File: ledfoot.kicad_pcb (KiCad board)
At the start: 2 copper layers, 29 x 84 mm, 24 parts, among them J1 1729144, J2 54-00167, J3 Conn_01x12_Pin, SW1 SW_Push, SW2 SW_Push, U1 MP1584EN, U2 SN74LVC1T45DBV

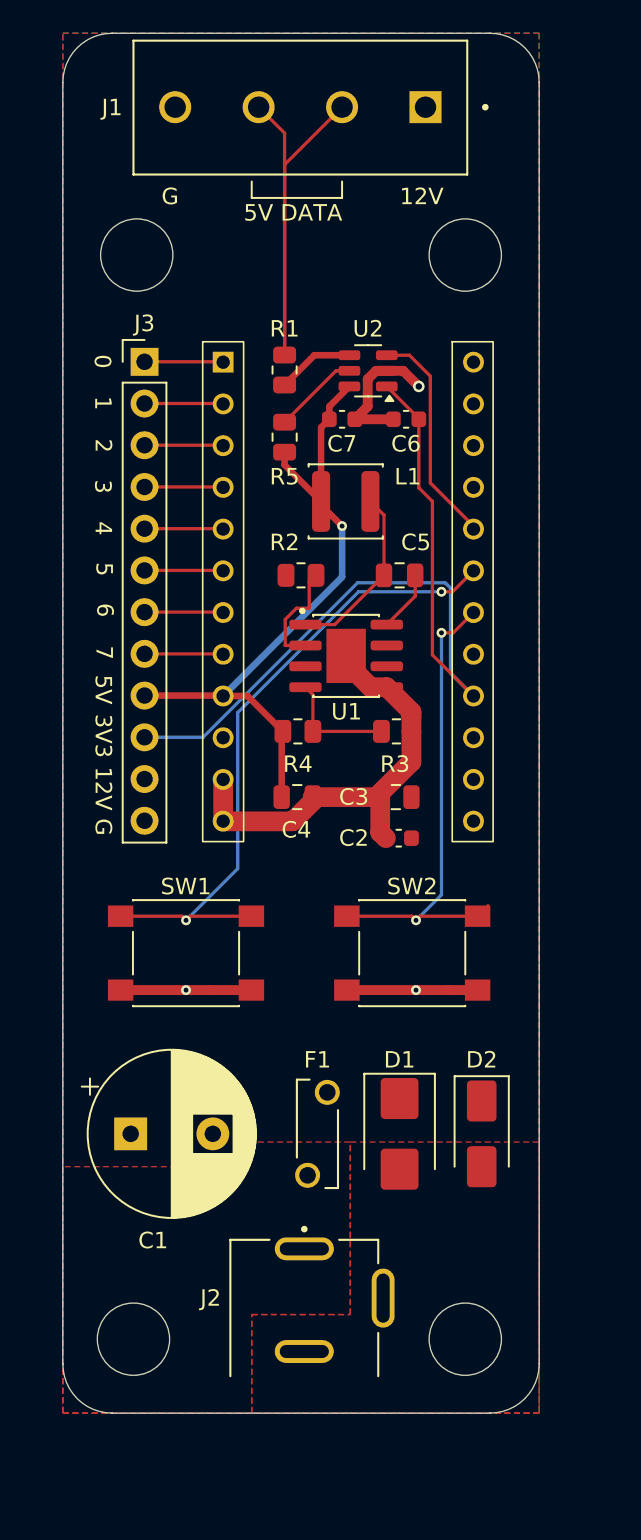
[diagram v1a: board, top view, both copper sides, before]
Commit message: Revision 2 ready for production
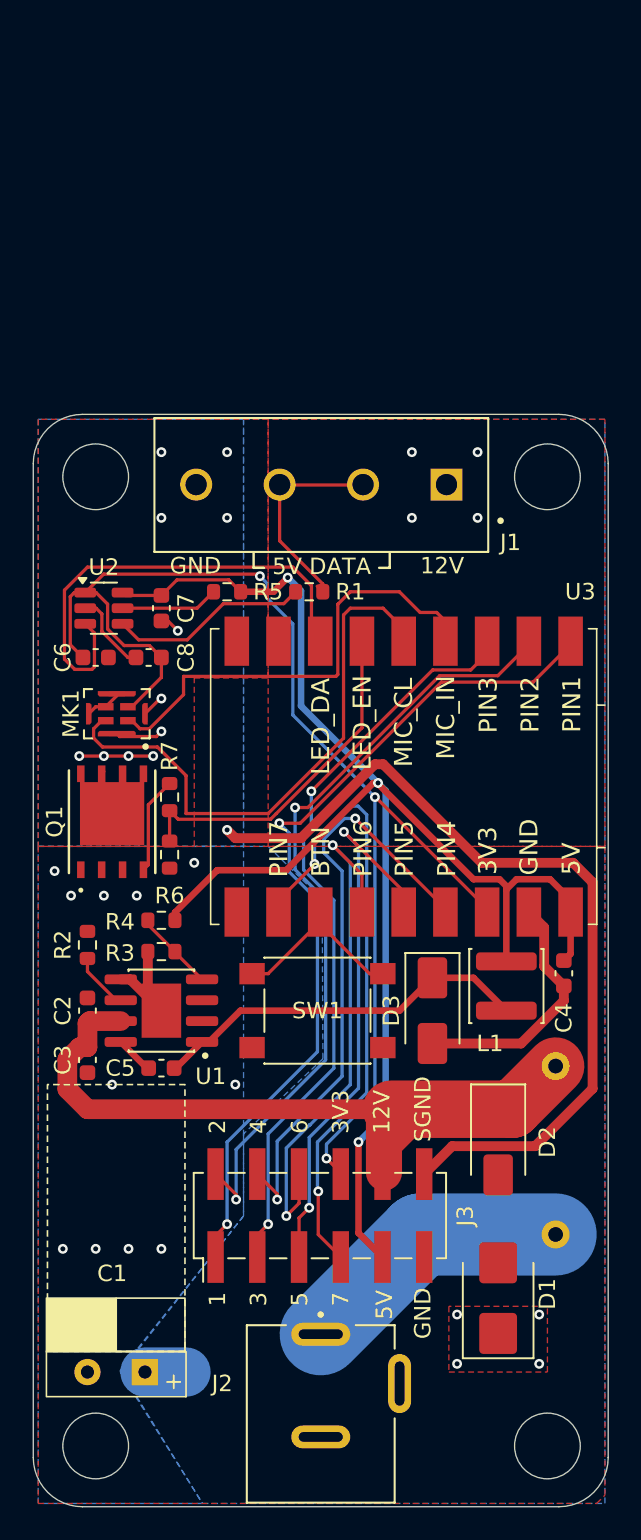
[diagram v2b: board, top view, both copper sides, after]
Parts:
- removed 1: U?, Custom:WeAct-ESP32C3CoreBoard
- removed SW2: SW_Push, Button_Switch_SMD:SW_SPST_PTS645
- added C8: 0.1µF, Capacitor_SMD:C_0603_1608Metric, F.Cu at (125.2, 85.0)
- added D3: SS34, Diode_SMD:D_SMA, F.Cu at (142.5, 106.5)
- added MK1: SPK0641HT4H-1, MIC_SPK0641HT4H-1:MIC_SPK0641HT4H-1, F.Cu at (123.3, 88.4)
- added Q1: SIRA20DP-T1-RE3, POWERPAK_SO-8_SINGLE_VIS:POWERPAK_SO-8_SINGLE_VIS, F.Cu at (123.0, 95.0)
- added R6: 1MΩ, Resistor_SMD:R_0603_1608Metric, F.Cu at (126.5, 97.0)
- added R7: 10Ω, Resistor_SMD:R_0603_1608Metric, F.Cu at (126.5, 93.5)
- added U3: ~, Tenstar-ESP32:Tenstar-ESP32-S3-SuperMini-EdgeOnly, F.Cu at (145.5, 91.8)
- C1: footprint Capacitor_THT:CP_Radial_D10.0mm_P5.00mm -> Capacitor_THT:CP_Radial_D8.0mm_P3.50mm
- C3, C4, C5: footprint Capacitor_SMD:C_0805_2012Metric -> Capacitor_SMD:C_0603_1608Metric
- D1: value SMBJ12A -> SMBJ13A
- F1: value 8A (RUEF800) -> 8A; footprint footprints:FUSRR505W81L660T250H1360 -> RUEF800:FUSE_RUEF800; moved to B.Cu
- J1: footprint footprints:PHOENIX_1729144 -> Phoenix:PHOENIX_1729144
- J2: footprint footprints:TENSILITY_54-00167 -> Tensility:TENSILITY_54-00167
- J3: value Conn_01x12_Pin -> Conn_02x05_Counter_Clockwise; footprint Connector_PinHeader_2.54mm:PinHeader_1x12_P2.54mm_Vertical -> Connector_PinHeader_2.54mm:PinHeader_2x06_P2.54mm_Vertical_SMD
- R1, R5: footprint Resistor_SMD:R_0805_2012Metric -> Resistor_SMD:R_0603_1608Metric
- R2: value 10kΩ -> 100kΩ; footprint Resistor_SMD:R_0805_2012Metric -> Resistor_SMD:R_0603_1608Metric
- R3: value 3.3kΩ -> 43kΩ; footprint Resistor_SMD:R_0805_2012Metric -> Resistor_SMD:R_0603_1608Metric
- R4: value 10kΩ -> 8.2kΩ; footprint Resistor_SMD:R_0805_2012Metric -> Resistor_SMD:R_0603_1608Metric
- U1: footprint Custom:SOIC127P600X170-9N -> MP1584EN:SOIC127P600X170-9N
- moved J3 53.1 mm to (135.7, 119.0), turned to 90 degrees
- moved C5 33.3 mm to (126.0, 110.0), turned to 0 degrees
- moved L1 31.1 mm to (147.0, 105.0), turned to 90 degrees
- moved R2 26.0 mm to (121.5, 102.5), turned to -90 degrees
- moved C3 24.7 mm to (121.5, 109.5), turned to 90 degrees
- moved U1 24.3 mm to (126.0, 106.5), turned to 180 degrees
- moved C6 23.8 mm to (122.0, 85.0), turned to 0 degrees
- moved J1 23.0 mm to (145.9, 70.4)
- moved C2 21.7 mm to (121.5, 106.5), turned to 90 degrees
- moved U2 21.6 mm to (122.5, 82.0), turned to 0 degrees
- moved R3 19.6 mm to (126.0, 102.9), turned to 180 degrees
- moved C4 19.5 mm to (150.5, 104.2), turned to 90 degrees
- moved C7 15.9 mm to (126.0, 82.0), turned to -90 degrees
- moved C1 14.5 mm to (125.0, 128.5), turned to 180 degrees
- moved R4 14.2 mm to (126.0, 101.0), turned to 0 degrees
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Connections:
- C6 pad 2: GND -> SGND
- C7 pad 2: GND -> SGND
- F1 pad 1: +12V -> 12V
- F1 pad 2: 12V -> +12V
- J1 pad 4: GND -> SGND
- J3 pad 1: Net-(1-IO0) -> PIN1
- J3 pad 10: 3V3 -> 12V
- J3 pad 11: 12V -> GND
- J3 pad 12: GND -> SGND
- J3 pad 2: Net-(1-IO1) -> PIN2
- J3 pad 3: Net-(1-IO2) -> PIN3
- J3 pad 4: Net-(1-IO3) -> PIN4
- J3 pad 5: Net-(1-IO4) -> PIN5
- J3 pad 6: Net-(1-IO5) -> PIN6
- J3 pad 7: Net-(1-IO6) -> PIN7
- J3 pad 8: Net-(1-IO7) -> 3V3
- R2 pad 1: 12V -> GND
- R2 pad 2: Net-(U1-EN) -> Net-(U1-FREQ)
- U1 pad 2: Net-(U1-EN) -> unconnected-(U1-EN-Pad2)
- U1 pad 6: unconnected-(U1-FREQ-Pad6) -> Net-(U1-FREQ)
- U2 pad 2: GND -> SGND
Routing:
- net SGND: track 0.00 -> 69.9 mm, vias 0 -> 12
- net 12V: track 0.07 -> 62.7 mm, vias 0 -> 8
- net 5V: track 40.4 -> 96.0 mm, vias 1 -> 3
- net PIN1: track 0.00 -> 52.4 mm, vias 0 -> 2
- net PIN2: track 0.00 -> 48.3 mm, vias 0 -> 2
- net PIN3: track 0.00 -> 46.2 mm, vias 0 -> 2
- net PIN7: track 0.00 -> 39.0 mm, vias 0 -> 2
- net PIN4: track 0.00 -> 36.5 mm, vias 0 -> 2
- net MIC_CLK: track 0.00 -> 34.5 mm
- net PIN5: track 0.00 -> 34.1 mm, vias 0 -> 2
- net PIN6: track 0.00 -> 32.9 mm, vias 0 -> 2
- net GND: track 53.1 -> 22.6 mm, vias 3 -> 11
- net Net-(1-IO8): track 29.7 -> 0.00 mm, vias 2 -> 0
- net Net-(U3-GP10): track 40.0 -> 11.8 mm, vias 2 -> 0
- net MIC_DATA: track 0.00 -> 28.1 mm
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- added copper zone on B.Cu, net 12V
- added copper zone on B.Cu, net SGND
- added copper zone on F.Cu, net SGND
- removed copper zone on F.Cu, net +12V
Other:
- board size 29 x 84 mm -> 35 x 66.5 mm
- board text added: "1"
- board text added: "2"
- board text added: "3"
- board text added: "3V3"
- board text added: "4"
- board text added: "5"
- board text added: "5V"
- board text added: "6"
- board text added: "7"
- board text added: "BTN"
- board text added: "GND"
- board text added: "LEDFoot rev. 2"
- board text added: "LED_DA"
- board text added: "LED_EN"
- board text added: "MIC_CL"
- board text added: "MIC_IN"
- board text added: "PIN1"
- board text added: "PIN2"
- board text added: "PIN3"
- board text added: "PIN4"
- board text added: "PIN5"
- board text added: "PIN6"
- board text added: "PIN7"
- board text added: "SGND"
- board text removed: "G"
- board text removed: "LEDFoot rev. 1"
